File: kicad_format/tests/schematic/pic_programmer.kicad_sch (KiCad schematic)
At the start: 56 parts, among them J1 DB9-FEMAL, P1 CONN_2, P101 CONN_1, P102 CONN_1, P103 CONN_1, P104 CONN_1, P105 CONN_1, P106 CONN_1, Q1 BC237, Q2 BC307, Q3 BC307, U2 74HC125, U3 7805, U4 LT1373

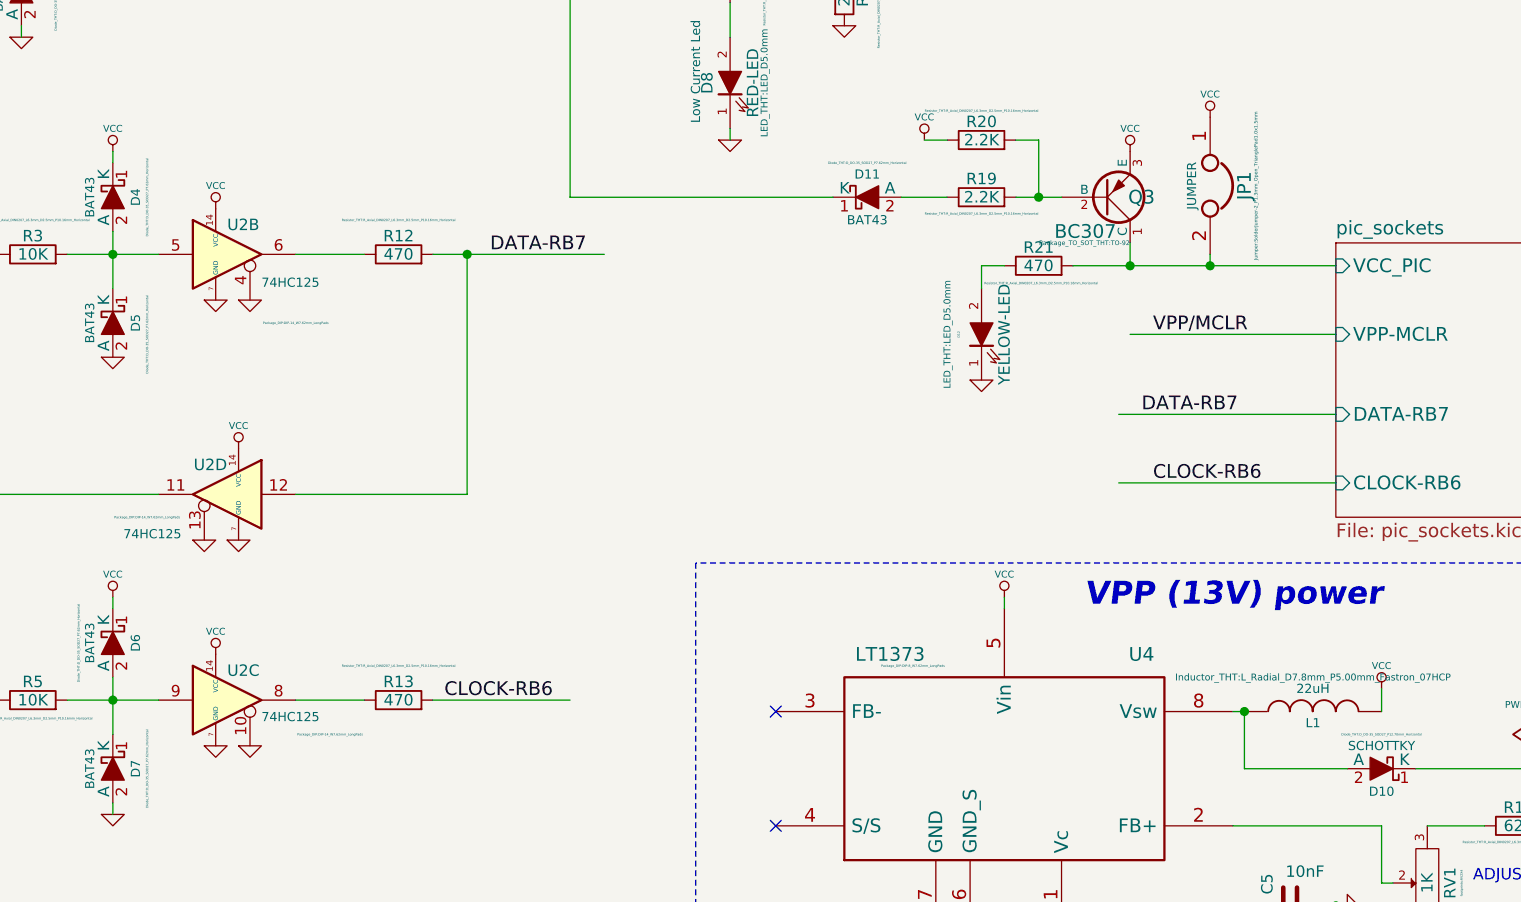
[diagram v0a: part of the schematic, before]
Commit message: kicad9
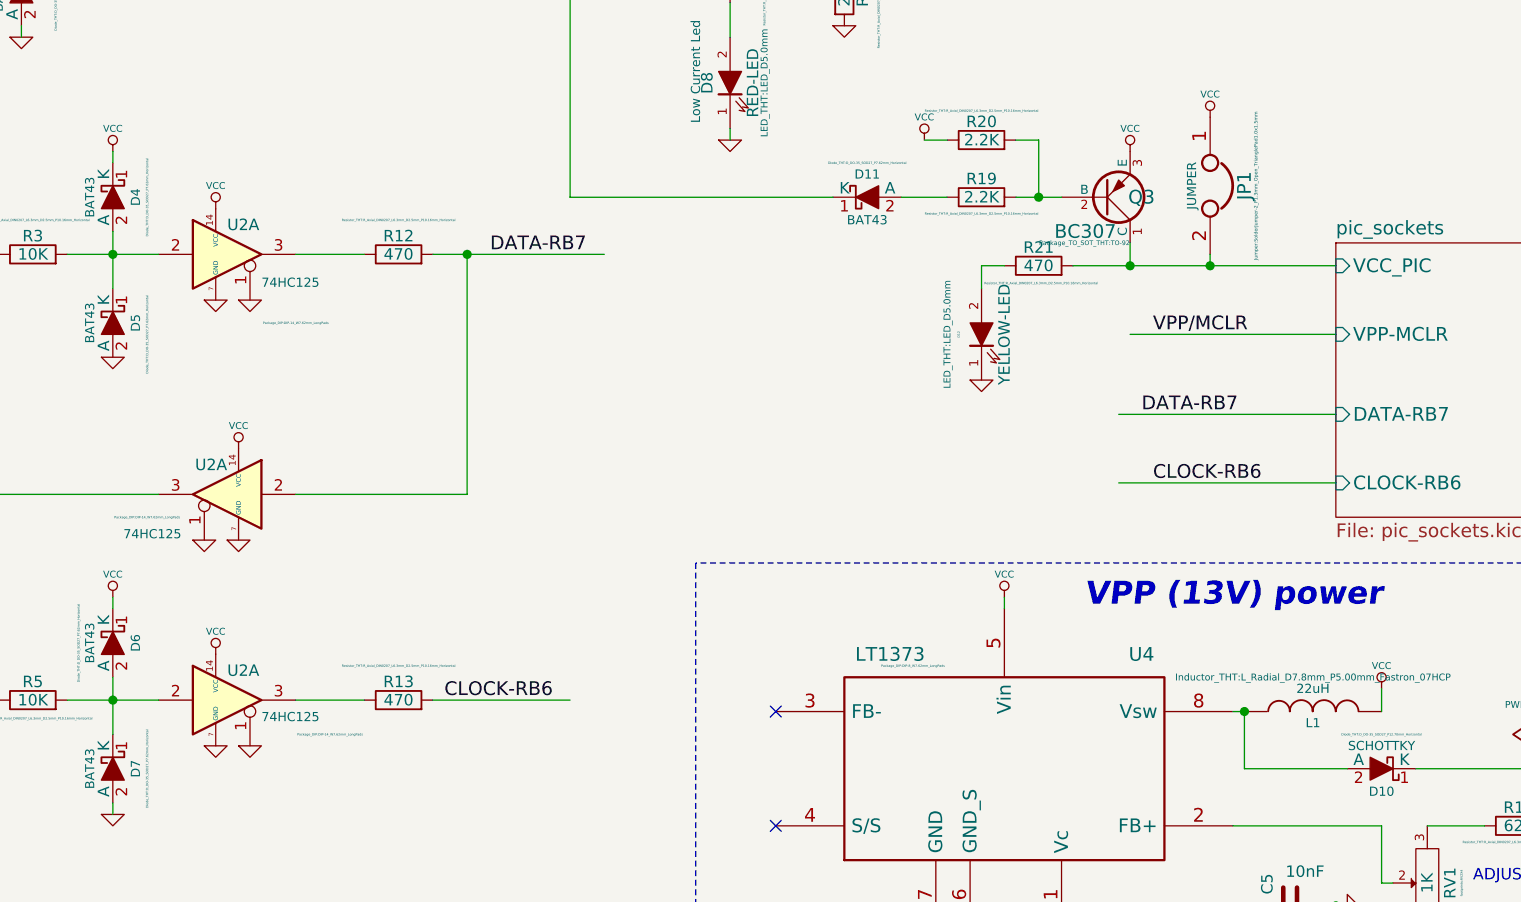
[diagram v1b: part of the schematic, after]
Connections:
- net DATA-RB7: now also U2.2; no longer U2.12
- net GND: now also U2.1, U2.1, U2.1; no longer U2.10, U2.13, U2.4
- net PC-DATA-IN: now also U2.3; no longer U2.11
- net at D4.2 (A), D5.1 (K), R3.2: now also U2.2; no longer U2.5
- net at R12.1: now also U2.3; no longer U2.6
- net at R13.1: now also U2.3; no longer U2.8
- net at D6.2 (A), D7.1 (K), R5.2: now also U2.2; no longer U2.9

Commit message: Revert "kicad9"
This reverts commit fe8acb19a57653eb9f4c3e1a43f922b9fa6082d1.
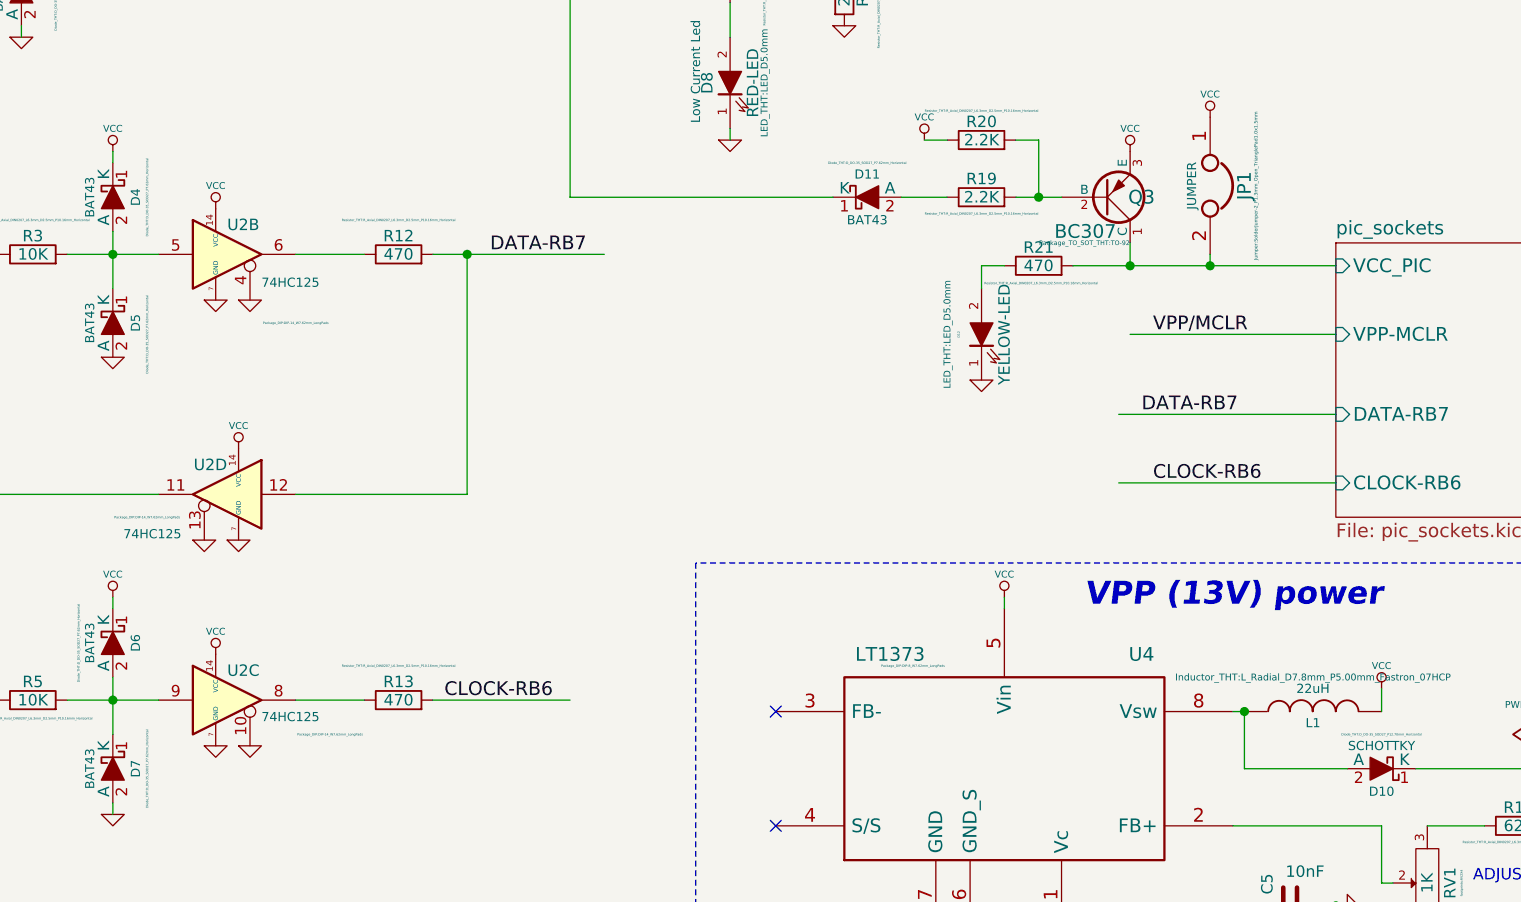
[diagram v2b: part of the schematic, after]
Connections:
- net DATA-RB7: now also U2.12; no longer U2.2
- net GND: now also U2.10, U2.13, U2.4; no longer U2.1, U2.1, U2.1
- net PC-DATA-IN: now also U2.11; no longer U2.3
- net at D4.2 (A), D5.1 (K), R3.2: now also U2.5; no longer U2.2
- net at R12.1: now also U2.6; no longer U2.3
- net at D6.2 (A), D7.1 (K), R5.2: now also U2.9; no longer U2.2
- net at R13.1: now also U2.8; no longer U2.3
